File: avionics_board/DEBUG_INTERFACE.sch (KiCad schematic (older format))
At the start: 25 parts, among them J12 Conn_01x05, J13 Conn_01x04_Male

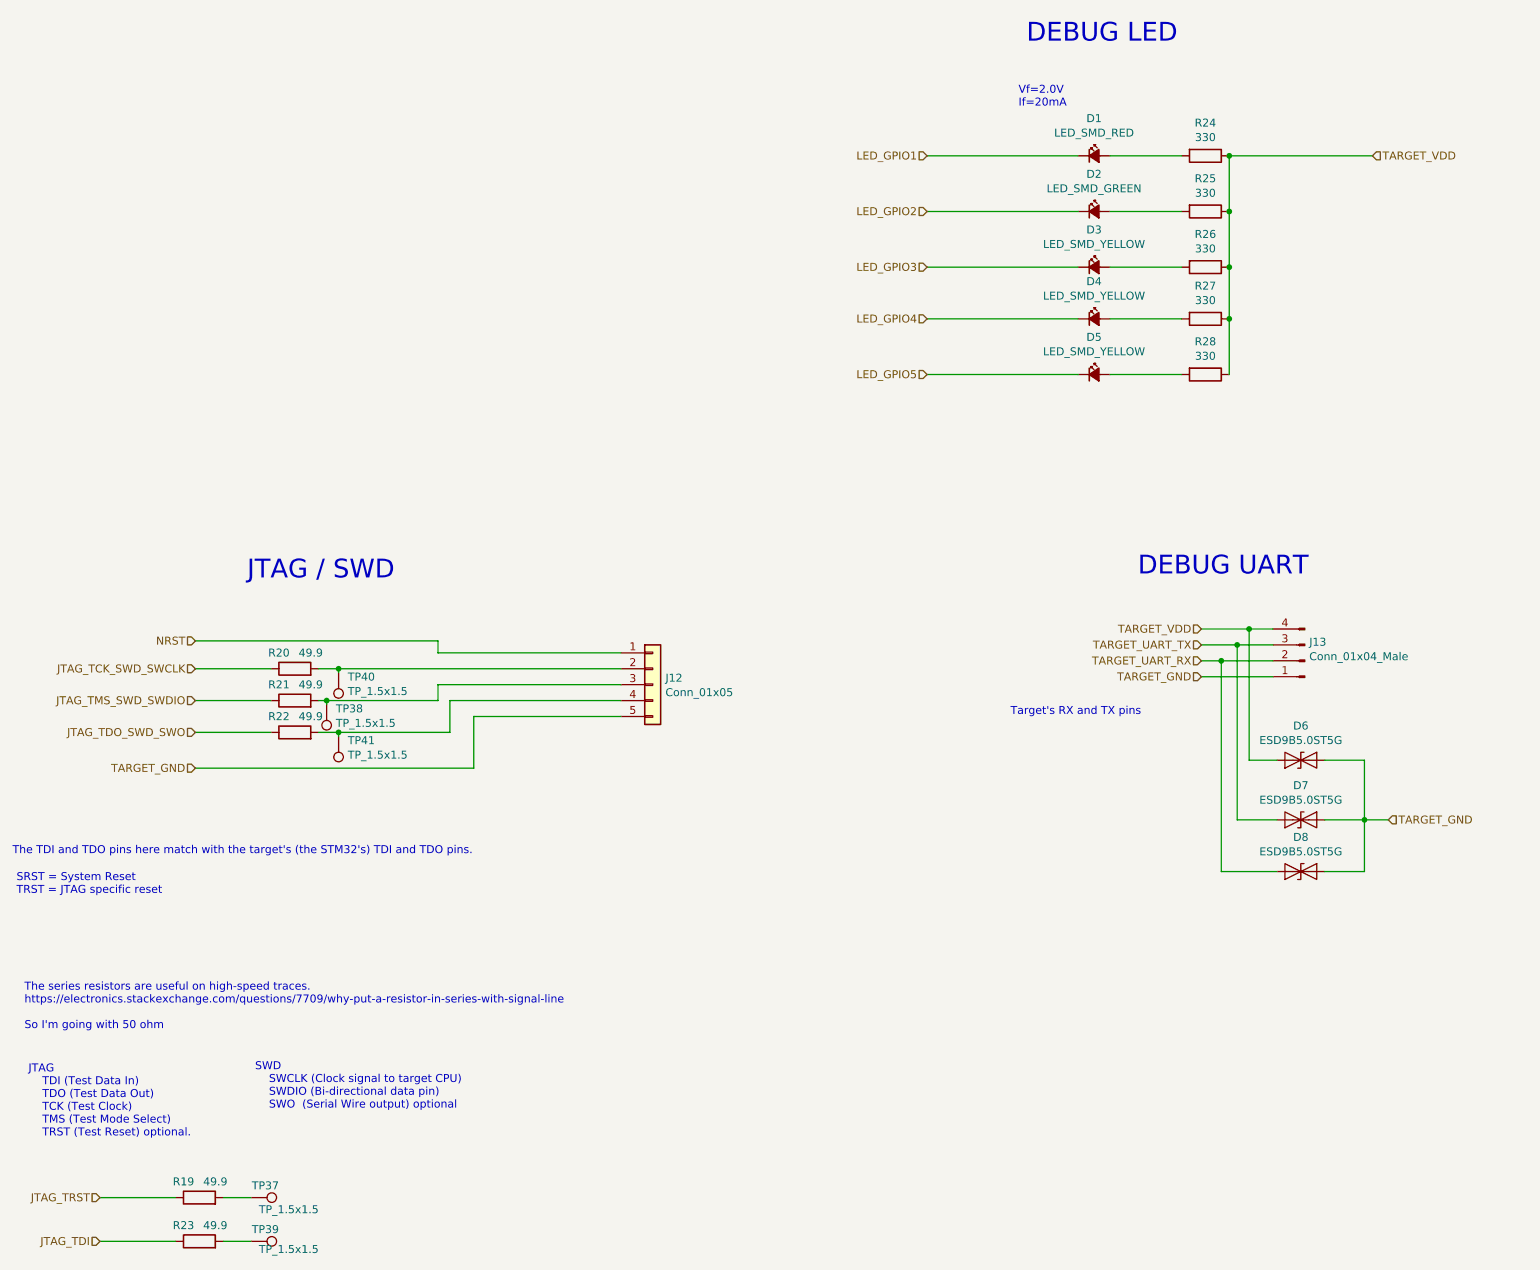
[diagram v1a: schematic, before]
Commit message: Essentially done with EPS schematic
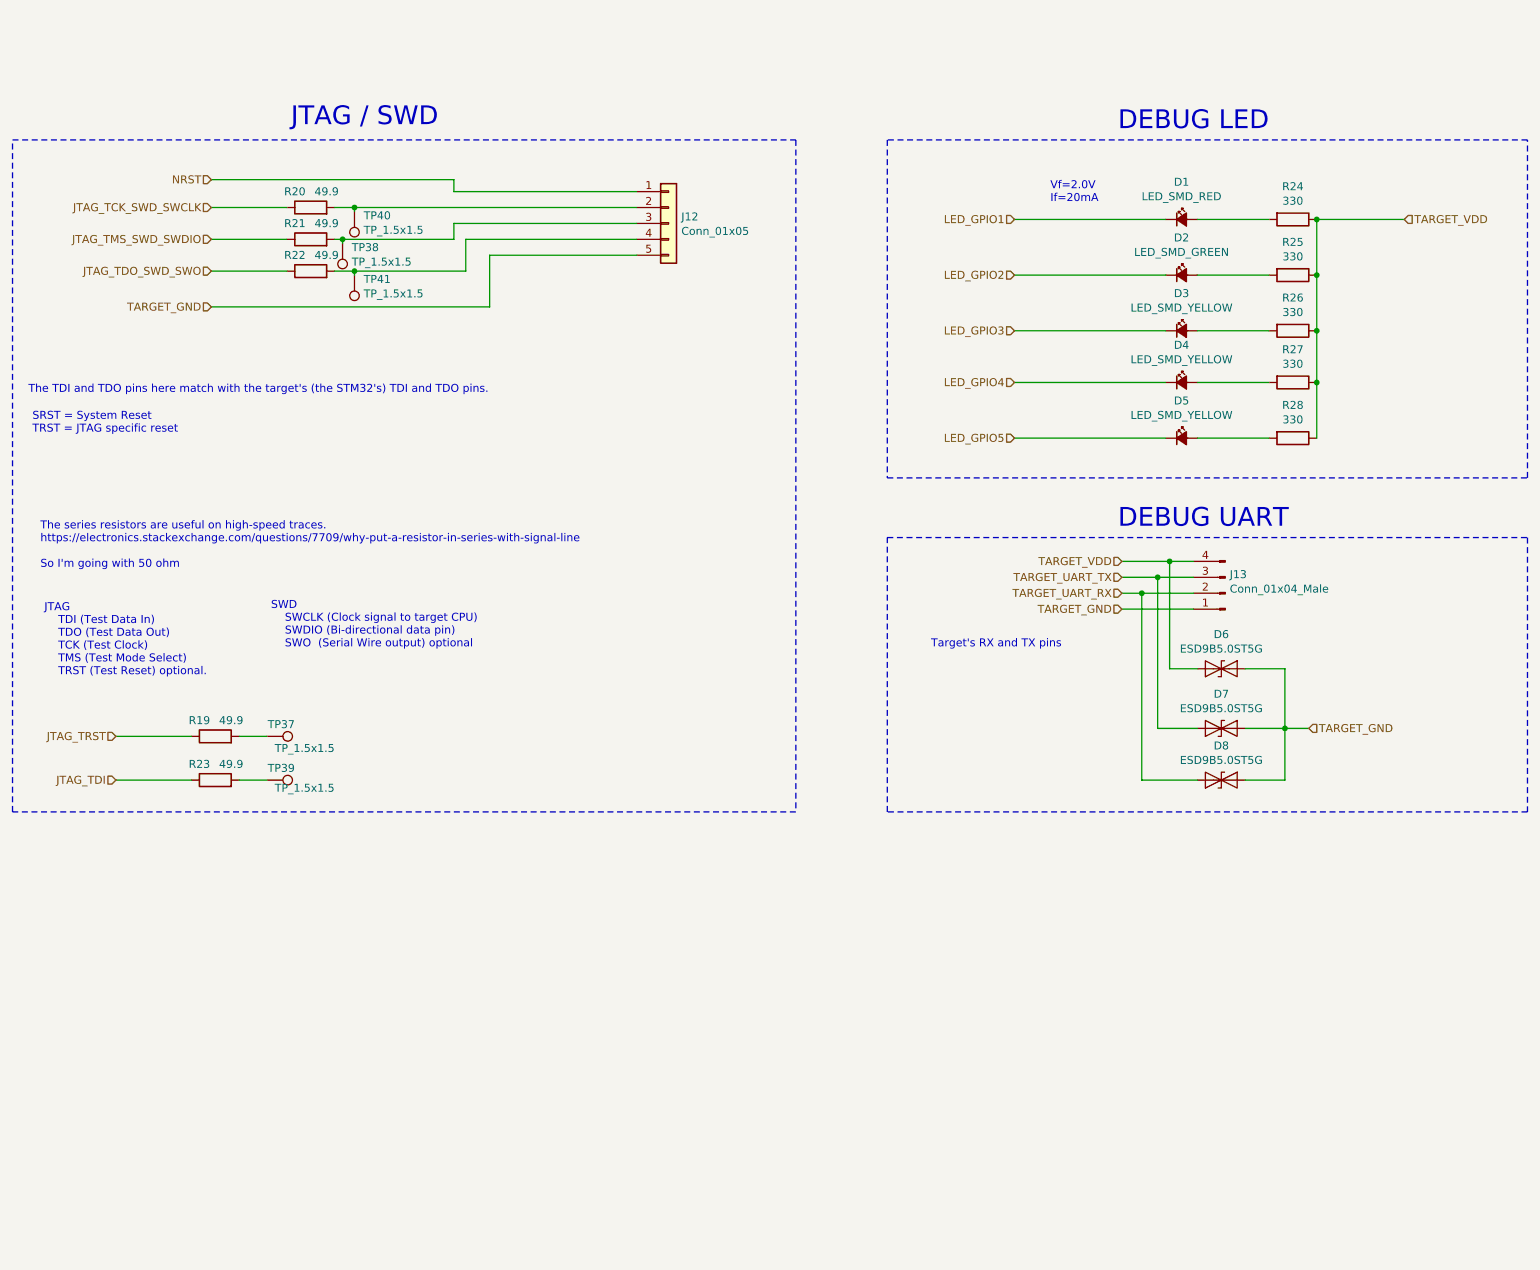
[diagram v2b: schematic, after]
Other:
- moved on the sheet: D1, D2, D3, D4, D5, D6, D7, D8, J12, J13, R19, R20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
